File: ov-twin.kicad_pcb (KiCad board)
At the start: 4 copper layers, 64 x 64 mm, 113 parts, among them J1 USB_C_Receptacle_USB2.0, J2 Conn_01x02, J3 Conn_01x02, SW1 SW_SPST, SW2 SW_SPST, SW3 SW_SPST, SW4 SW_SPST, SW5 SW_SPST, SW6 SW_SPST, SW7 SW_SPST, SW8 SW_SPST, U1 NCP1117-3.3_SOT223, U2 RP2040, U3 RP2040, U4 W25Q128JVS, U5 W25Q128JVS, U7 LIS3DH, U8 SN74LVC1T45DBV, Y1 Crystal_GND24, Y2 Crystal_GND24, Y3 Crystal_GND24

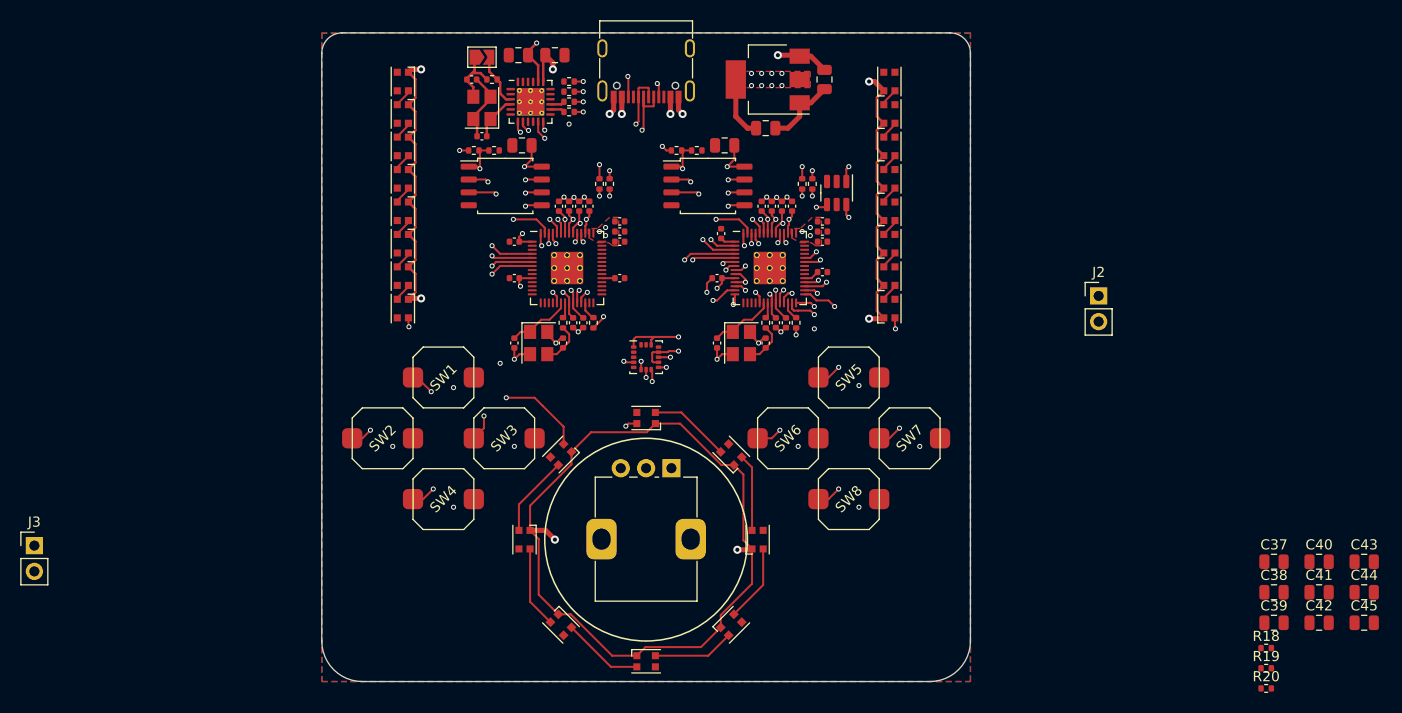
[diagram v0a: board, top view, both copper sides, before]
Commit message: That worked pretty well I thought!
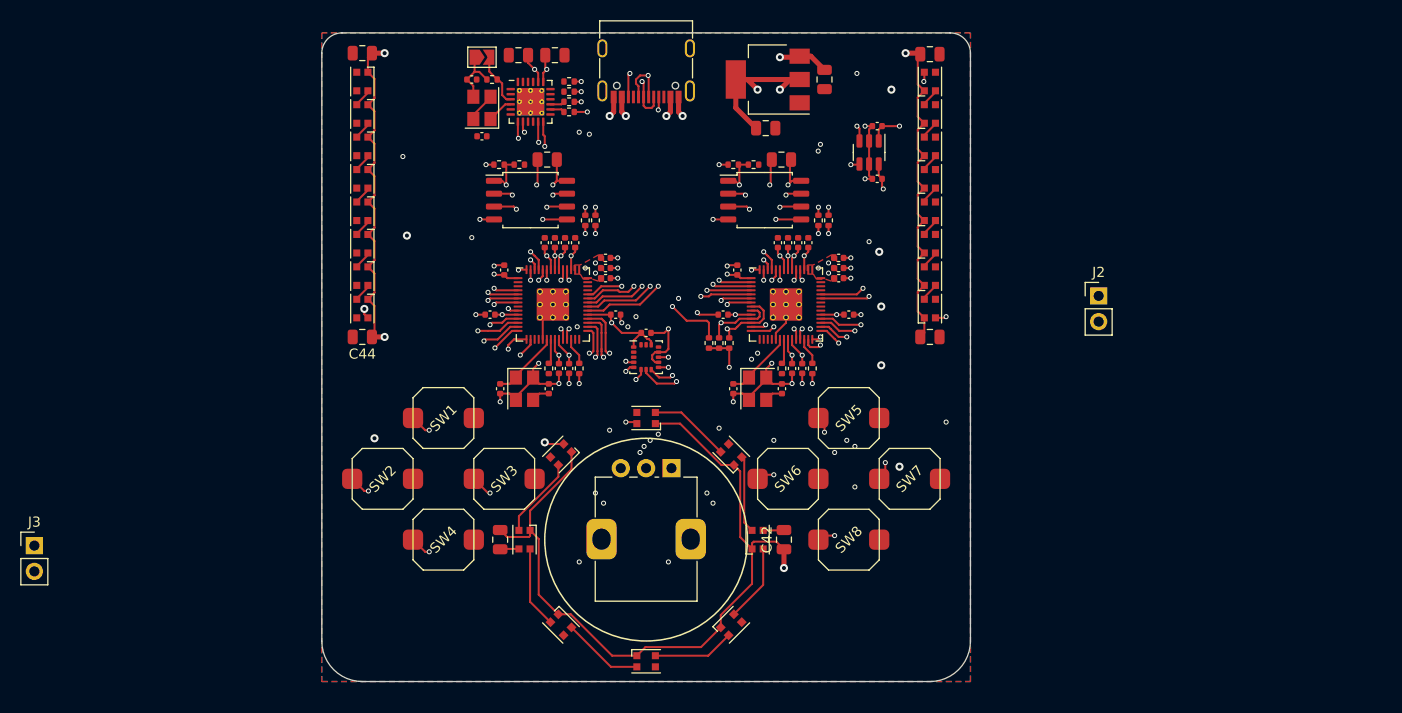
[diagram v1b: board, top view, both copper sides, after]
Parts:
- C37, C38, C39: footprint Capacitor_SMD:C_0805_2012Metric -> Capacitor_SMD:C_0402_1005Metric
- moved C45 113.7 mm to (144.0, 62.0), turned to 180 degrees
- moved C44 102.0 mm to (144.0, 90.0), turned to 180 degrees
- moved C43 85.3 mm to (157.6, 110.0), turned to -90 degrees
- moved C37 65.9 mm to (172.0, 89.6), turned to 180 degrees
- moved R20 64.7 mm to (178.2, 90.6), turned to 90 degrees
- moved C40 63.1 mm to (200.0, 62.1)
- moved R19 62.8 mm to (179.2, 90.6), turned to 90 degrees
- moved C39 62.7 mm to (194.8, 69.2)
- moved R18 60.9 mm to (180.2, 90.6), turned to 90 degrees
- moved C38 56.5 mm to (194.8, 74.4)
- moved C42 53.4 mm to (185.6, 110.0), turned to 90 degrees
- moved C41 45.9 mm to (200.0, 90.0)
- moved C31 5.77 mm to (185.3, 72.5)
- moved R11 5.77 mm to (182.6, 73.0)
- moved R12 5.77 mm to (180.6, 73.0)
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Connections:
- C37 pad 1: +3V3 -> GND
- C37 pad 2: GND -> +3V3
- C38 pad 1: +3V3 -> GND
- C38 pad 2: GND -> +3V3
- C39 pad 1: +5V -> GND
- C39 pad 2: GND -> +5V
- U2 pad 11: unconnected-(U2-GPIO8-Pad11) -> /lis3dh-int1
- U2 pad 17: /lis3dh-sdi-sda -> unconnected-(U2-GPIO14-Pad17)
- U2 pad 18: /lis3dh-scl-spc -> unconnected-(U2-GPIO15-Pad18)
- U2 pad 27: /lis3dh-int2 -> unconnected-(U2-GPIO16-Pad27)
- U2 pad 28: /lis3dh-int1 -> unconnected-(U2-GPIO17-Pad28)
- U2 pad 29: /pi-b-sw-1 -> /pi-b-sw-4
- U2 pad 30: /pi-b-sw-2 -> /pi-b-sw-3
- U2 pad 31: /pi-b-sw-3 -> /pi-b-sw-2
- U2 pad 32: /pi-b-sw-4 -> /pi-b-sw-1
- U2 pad 9: unconnected-(U2-GPIO7-Pad9) -> /lis3dh-int2
- U8 pad 2: Net-(U8-DIR) -> GND
- U8 pad 3: /smartled-5v -> /smartled-5v0
- U8 pad 5: Net-(U8-DIR) -> GND
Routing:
- net +3V3: track 79.3 -> 375.6 mm, vias 33 -> 36
- net /smartled-3v3: track 8.34 -> 73.4 mm, vias 2 -> 5
- net /pi-b-sw-8: track 25.3 -> 71.0 mm, vias 2 -> 5
- net /pi-b-sw-6: track 19.2 -> 60.6 mm, vias 2 -> 6
- net /pi-b-sw-5: track 12.2 -> 53.0 mm, vias 2 -> 4
- net /pi-b-sw-4: track 43.8 -> 83.3 mm, vias 2 -> 5
- net /pi-b-sw-7: track 25.8 -> 64.0 mm, vias 2 -> 5
- net /pi-b-sw-2: track 46.3 -> 81.5 mm, vias 2 -> 5
- net /pi-b-sw-3: track 35.4 -> 65.4 mm, vias 2 -> 5
- net /lis3dh-cs: track 16.7 -> 46.0 mm, vias 2 -> 4
- net /lis3dh-sdo-sa0: track 16.6 -> 45.6 mm, vias 2 -> 4
- net /lis3dh-int2: track 13.0 -> 41.2 mm, vias 2 -> 4
- net /pi-b-pot: track 41.3 -> 69.4 mm, vias 1 -> 3
- net /lis3dh-int1: track 11.9 -> 38.7 mm, vias 2 -> 4
- net GND: track 49.3 -> 73.4 mm, vias 26 -> 30
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- removed copper zone on In2.Cu, net +3V3
